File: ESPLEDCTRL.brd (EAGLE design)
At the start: 102.5 x 80 mm, 6 parts, among them J1 22-27-2031-03, X3 ZX62D-B-5PA8

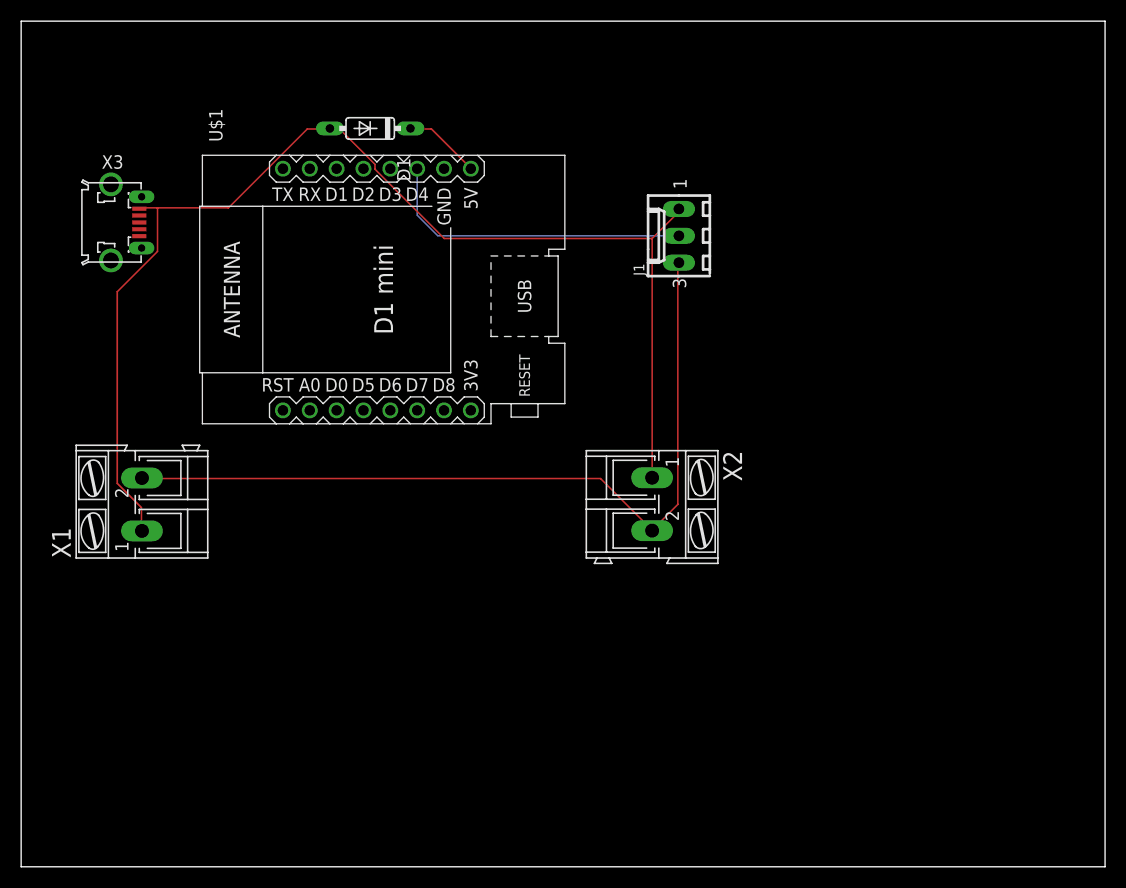
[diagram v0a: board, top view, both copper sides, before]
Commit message: Alte Version
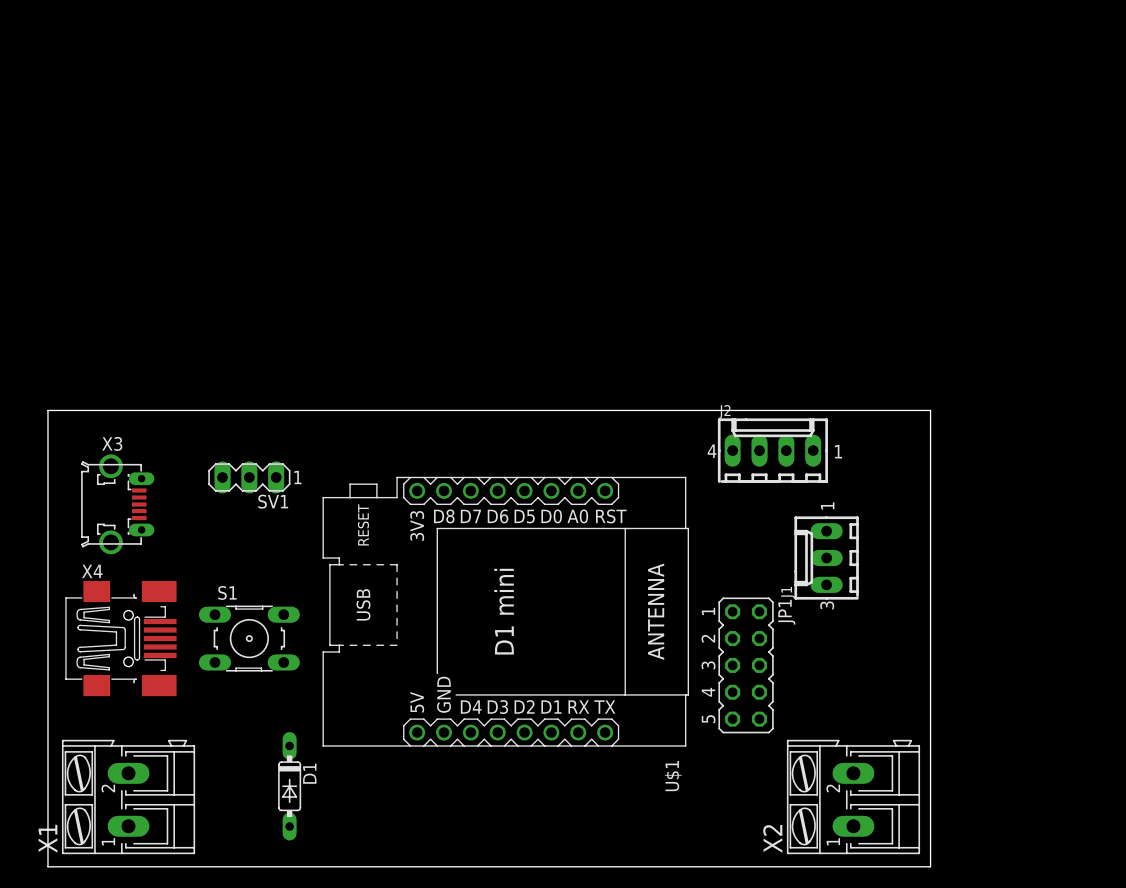
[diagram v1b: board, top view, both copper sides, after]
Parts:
- added J2: 22-27-2041-04, con-molex:6410-04
- added JP1: (no value), jumper:JP5Q
- added S1: (no value), switch-omron:B3F-10XX
- added SV1: (no value), con-lstb:MA03-1
- added X4: MINI-USB-32005-201, con-cypressindustries:32005-201
- moved D1 62.7 mm to (22.9, 7.62), turned to 270 degrees
- moved X2 33.8 mm to (76.2, 6.35), turned to 90 degrees
- moved J1 33.5 mm to (73.7, 29.2)
- moved U$1 32.6 mm to (43.2, 24.1), turned to 270 degrees
- moved X1 28.0 mm to (7.62, 6.35)
- moved X3 26.7 mm to (3.81, 34.3)
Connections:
- removed net 3V3: U$1.JP1.8
- new net N$10: J2.3, U$1.JP1.2
- new net N$11: J1.3, J2.1, JP1.10, JP1.2, JP1.4, JP1.6, JP1.8, S1.3, X1.2, X2.2, X3.5, X4.5
- new net N$12: J2.4, U$1.JP1.8
- new net N$13: D1.A, J1.1, SV1.1, X1.1, X2.1, X3.1, X4.1
- new net N$14: SV1.3, X3.3
- new net N$5: JP1.1, U$1.JP2.4
- new net N$6: J2.2, U$1.JP1.1
- new net N$7: JP1.3, U$1.JP2.3
- new net N$8: JP1.5, U$1.JP2.2
- new net N$9: JP1.7, U$1.JP2.1
- net N$3: now also SV1.2, X3.2; no longer D1.A, J1.1, X1.1, X2.1, X3.1
- net N$4: now also JP1.9, S1.1, U$1.JP2.5; no longer J1.3, X1.2, X2.2
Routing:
- net N$3: track 115.9 -> 0.00 mm
- net N$4: track 76.8 -> 0.00 mm
- net N$1: track 30.0 -> 0.00 mm
- net N$2: track 7.33 -> 0.00 mm
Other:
- board size 102.5 x 80 mm -> 83.5 x 43.2 mm
